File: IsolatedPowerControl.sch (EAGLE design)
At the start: 38 parts, among them IC1 LM358, K2 G2RATE-OJ, Q1 FDN360P, U1 MCP23008-E/SO, U2 MCP4716A0T-E/CH

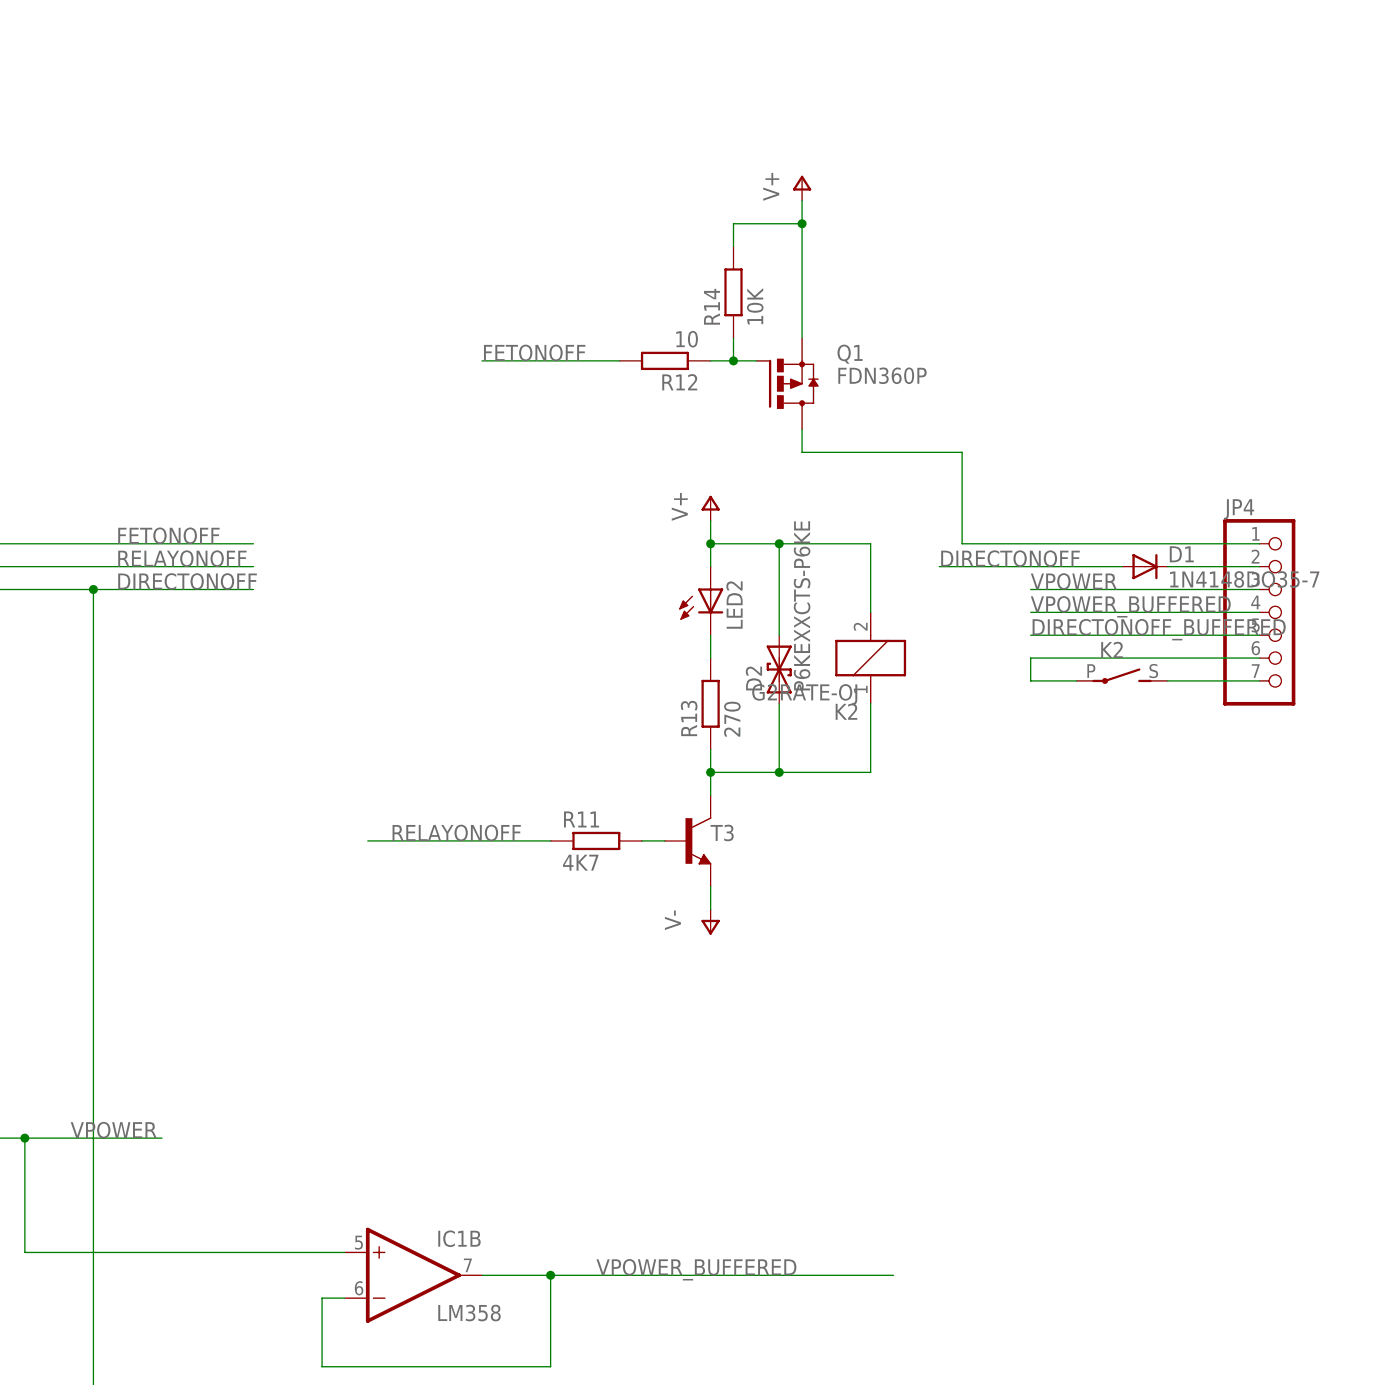
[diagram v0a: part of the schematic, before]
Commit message: Initial fit (incomplete routing)
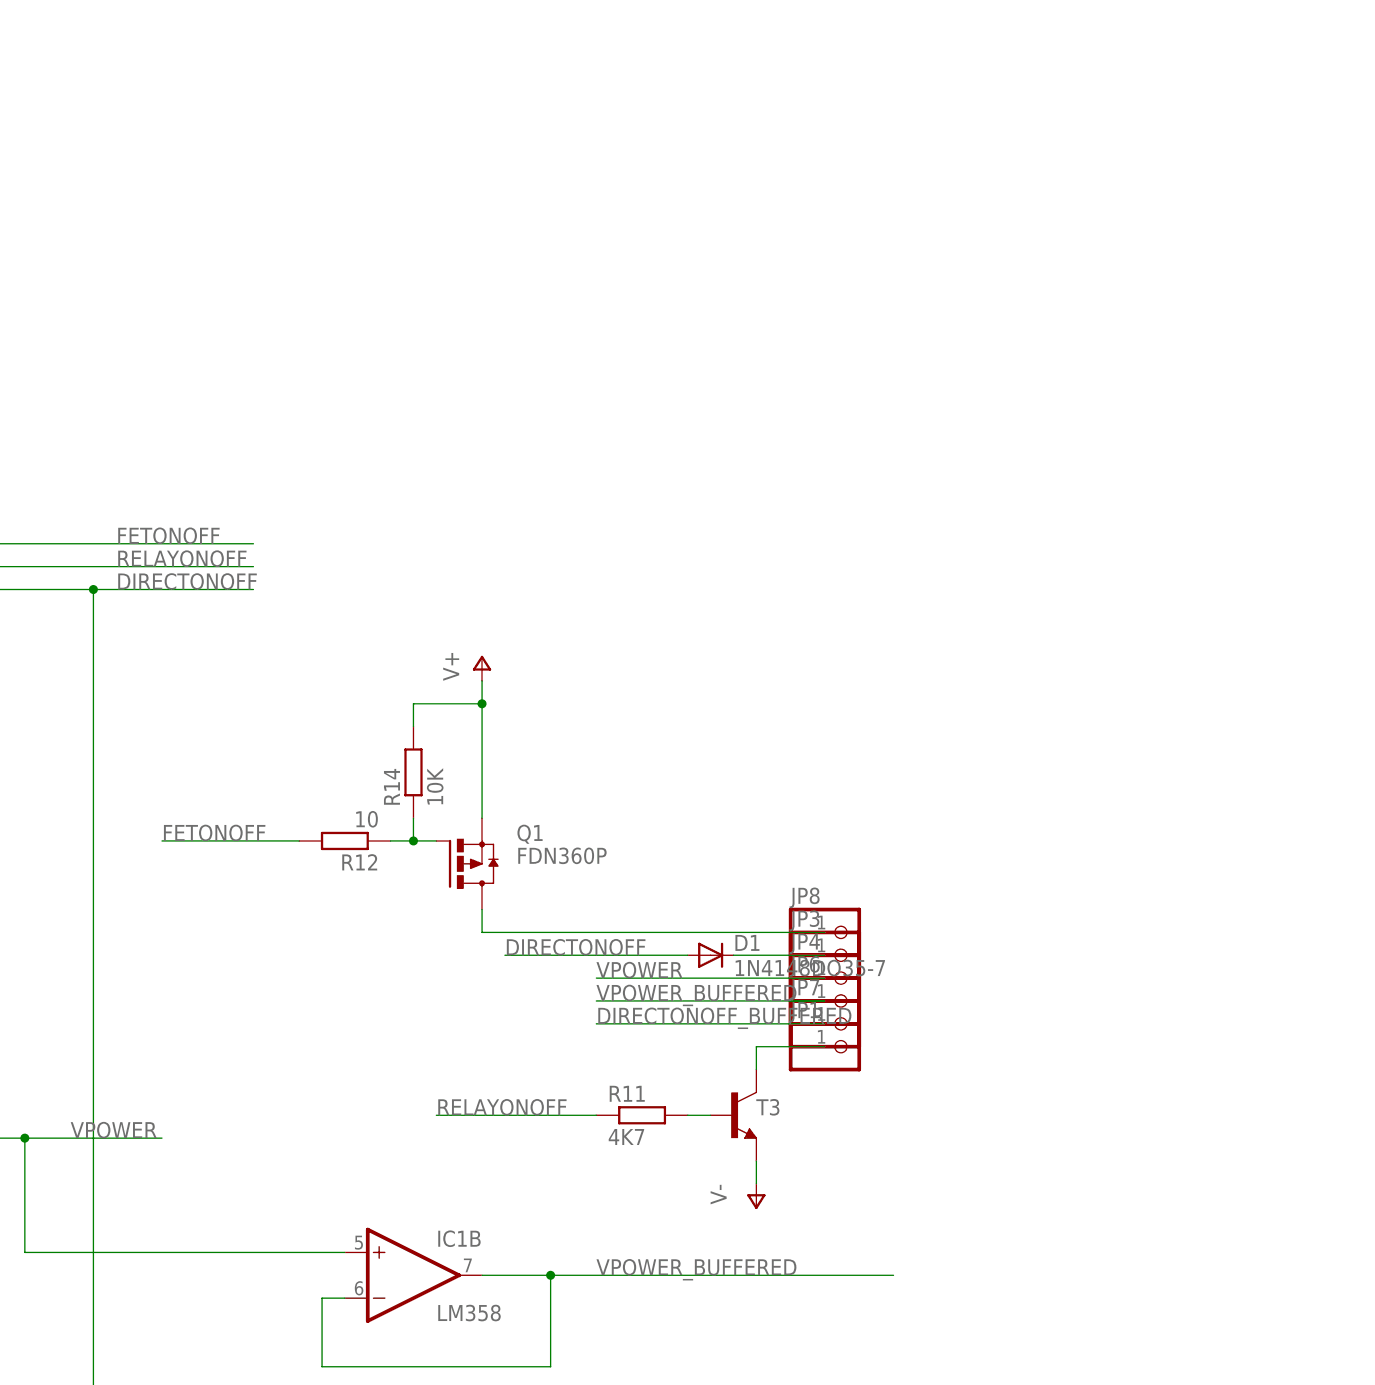
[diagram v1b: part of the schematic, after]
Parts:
- removed D2: P6KEXXCTS-P6KE, diode:P6KEXXCTS-P6KE
- removed K2: G2RATE-OJ, relay:G2RATE-OJ
- removed LED2: (no value), led:LED5MM
- removed R13: 270, rcl:R-EU_R0805
- added JP1, JP3, JP6, JP7, JP8: (no value), pinhead:PINHD-1X1
- JP4: device pinhead:PINHD-1X7 -> pinhead:PINHD-1X1
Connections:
- removed net N$10: JP4.7, K22.S
- removed net N$8: LED2.C, R13.2
- removed net N$9: JP4.6, K22.P
- net DIRECTONOFF_BUFFERED: now also JP7.1; no longer JP4.5
- net N$13: now also JP8.1; no longer JP4.1
- net N$18: now also JP1.1; no longer D2.1, K21.1, R13.1
- net N$3: now also JP3.1; no longer JP4.2
- net V+: no longer D2.2, K21.2, LED2.A
- net VPOWER: now also JP4.1; no longer JP4.3
- net VPOWER_BUFFERED: now also JP6.1; no longer JP4.4
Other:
- moved on the sheet: D1, Q1, R11, R12, R14, T3

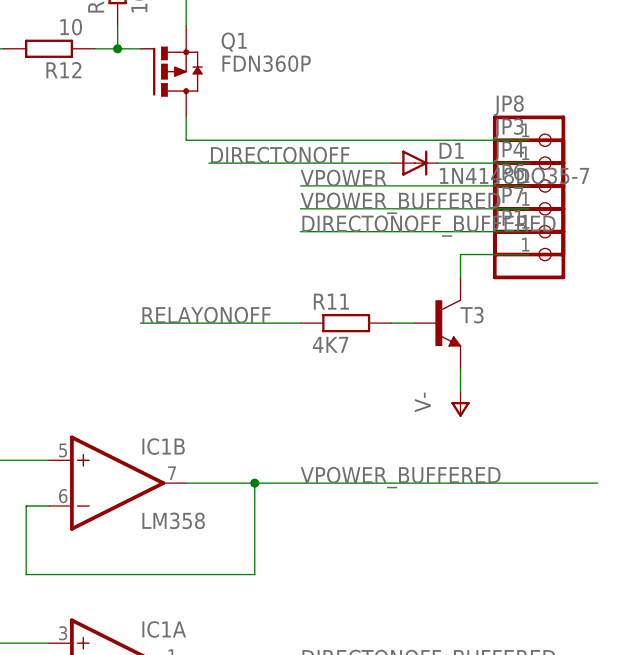
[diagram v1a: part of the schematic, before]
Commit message: First layout complete and checked
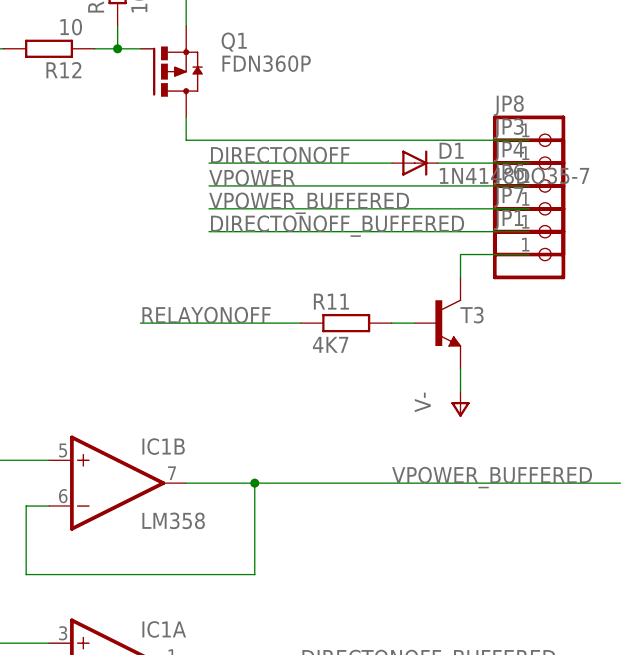
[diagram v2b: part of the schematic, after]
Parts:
- JP1, JP3, JP4, JP6, JP7, JP8: device pinhead:PINHD-1X1 -> pinhead:PINHD-1X1LARGEPAD
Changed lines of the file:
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@@
 <part name="JP5" library="pinhead" deviceset="PINHD-1X4" device=""/>
 <part name="JP2" library="pinhead" deviceset="PINHD-1X2" device=""/>
-<part name="JP1" library="pinhead" deviceset="PINHD-1X1" device=""/>
-<part name="JP3" library="pinhead" deviceset="PINHD-1X1" device=""/>
-<part name="JP4" library="pinhead" deviceset="PINHD-1X1" device=""/>
-<part name="JP6" library="pinhead" deviceset="PINHD-1X1" device=""/>
-<part name="JP7" library="pinhead" deviceset="PINHD-1X1" device=""/>
-<part name="JP8" library="pinhead" deviceset="PINHD-1X1" device=""/>
+<part name="JP1" library="pinhead" deviceset="PINHD-1X1" device="LARGEPAD"/>
+<part name="JP3" library="pinhead" deviceset="PINHD-1X1" device="LARGEPAD"/>
+<part name="JP4" library="pinhead" deviceset="PINHD-1X1" device="LARGEPAD"/>
+<part name="JP6" library="pinhead" deviceset="PINHD-1X1" device="LARGEPAD"/>
+<part name="JP7" library="pinhead" deviceset="PINHD-1X1" device="LARGEPAD"/>
+<part name="JP8" library="pinhead" deviceset="PINHD-1X1" device="LARGEPAD"/>
 </parts>
 <sheets>
@@
 </segment>
 <segment>
-<wire x1="347.98" y1="-40.64" x2="322.58" y2="-40.64" width="0.1524" layer="91"/>
-<label x="322.58" y="-40.64" size="1.778" layer="95"/>
+<wire x1="347.98" y1="-40.64" x2="312.42" y2="-40.64" width="0.1524" layer="91"/>
+<label x="312.42" y="-40.64" size="1.778" layer="95"/>
 <pinref part="JP4" gate="G$1" pin="1"/>
 </segment>
@@
 <net name="VPOWER_BUFFERED" class="0">
 <segment>
-<label x="322.58" y="-43.18" size="1.778" layer="95"/>
-<wire x1="347.98" y1="-43.18" x2="322.58" y2="-43.18" width="0.1524" layer="91"/>
+<label x="312.42" y="-43.18" size="1.778" layer="95"/>
+<wire x1="347.98" y1="-43.18" x2="312.42" y2="-43.18" width="0.1524" layer="91"/>
 <pinref part="JP6" gate="G$1" pin="1"/>
 </segment>
 <segment>
-<wire x1="309.88" y1="-73.66" x2="317.5" y2="-73.66" width="0.1524" layer="91"/>
+<label x="332.74" y="-73.66" size="1.778" layer="95"/>
+<wire x1="317.5" y1="-73.66" x2="358.14" y2="-73.66" width="0.1524" layer="91"/>
+<pinref part="IC1" gate="B" pin="OUT"/>
+<wire x1="317.5" y1="-73.66" x2="309.88" y2="-73.66" width="0.1524" layer="91"/>
 <wire x1="317.5" y1="-73.66" x2="317.5" y2="-83.82" width="0.1524" layer="91"/>
+<junction x="317.5" y="-73.66"/>
 <wire x1="317.5" y1="-83.82" x2="292.1" y2="-83.82" width="0.1524" layer="91"/>
 <wire x1="292.1" y1="-83.82" x2="292.1" y2="-76.2" width="0.1524" layer="91"/>
+<pinref part="IC1" gate="B" pin="-IN"/>
 <wire x1="292.1" y1="-76.2" x2="294.64" y2="-76.2" width="0.1524" layer="91"/>
-<wire x1="317.5" y1="-73.66" x2="355.6" y2="-73.66" width="0.1524" layer="91"/>
-<junction x="317.5" y="-73.66"/>
-<label x="322.58" y="-73.66" size="1.778" layer="95"/>
-<pinref part="IC1" gate="B" pin="-IN"/>
-<pinref part="IC1" gate="B" pin="OUT"/>
 </segment>
 </net>
@@
 </segment>
 <segment>
-<wire x1="347.98" y1="-45.72" x2="322.58" y2="-45.72" width="0.1524" layer="91"/>
-<label x="322.58" y="-45.72" size="1.778" layer="95"/>
+<wire x1="347.98" y1="-45.72" x2="312.42" y2="-45.72" width="0.1524" layer="91"/>
+<label x="312.42" y="-45.72" size="1.778" layer="95"/>
 <pinref part="JP7" gate="G$1" pin="1"/>
 </segment>
